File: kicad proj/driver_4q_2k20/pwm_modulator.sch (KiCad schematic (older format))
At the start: 9 parts, among them U2 LM555

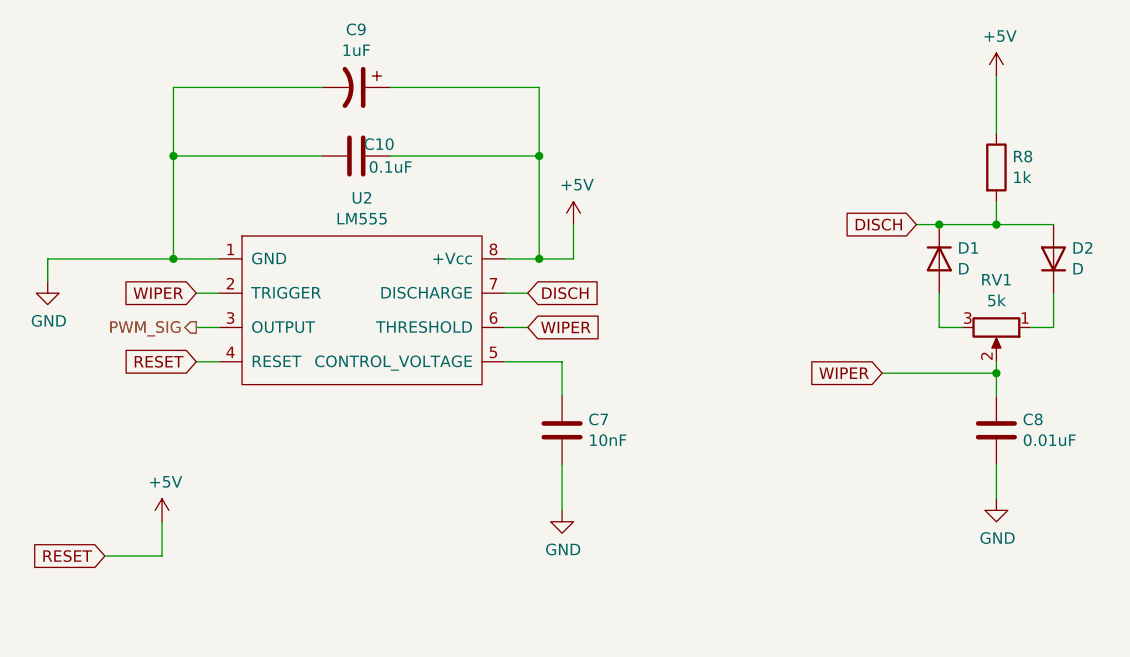
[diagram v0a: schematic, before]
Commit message: adicionado arquivos step, docs e footprints
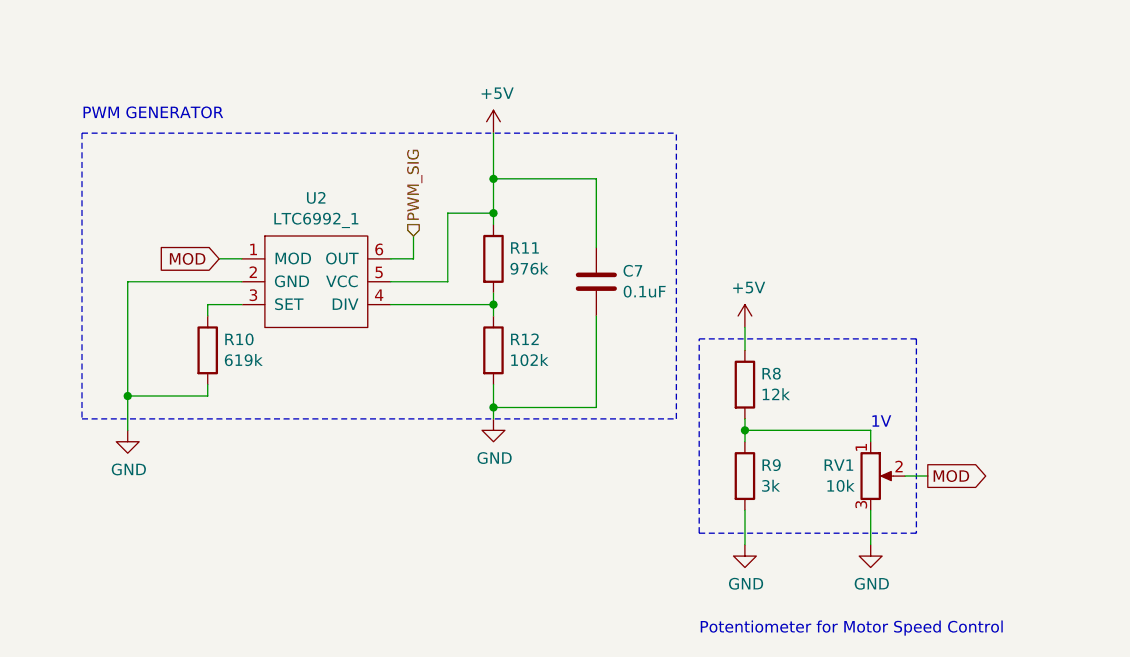
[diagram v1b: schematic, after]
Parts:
- removed C10: 0.1uF, driver_4q_2k20:C_0402_1005Metric, symbol Device:C
- removed C8: 0.01uF, driver_4q_2k20:C_0402_1005Metric, symbol Device:C
- removed C9: 1uF, driver_4q_2k20:CP_Radial_D5.0mm_P2.00mm, symbol Device:CP1
- removed D1, D2: D, driver_4q_2k20:S1_SMA, symbol Device:D
- removed U2: LM555, driver_4q_2k20:TI_DGN_S-PDSO-G8, symbol driver_4q_2k20_lib:555
- added R10: 619k, driver_4q_2k20:R_0402_1005Metric, symbol Device:R
- added R11: 976k, driver_4q_2k20:R_0402_1005Metric, symbol Device:R
- added R12: 102k, driver_4q_2k20:R_0402_1005Metric, symbol Device:R
- added R9: 3k, driver_4q_2k20:R_0402_1005Metric, symbol Device:R
- added U2: LTC6992_1, driver_4q_2k20:TSOT-23-6, symbol driver_4q_2k20_lib:LTC6992_1
- C7: value 10nF -> 0.1uF; Comment (none) -> ceramic / near LTC6992
- R8: value 1k -> 12k; footprint driver_4q_2k20:C_0402_1005Metric -> driver_4q_2k20:R_0402_1005Metric
- RV1: value 5k -> 10k
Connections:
- net DISCH is gone; now on an unnamed net: R8.2
- net +5V: now also C7.1, R11.1, U2.5 (VCC)
- net GND: now also RV1.3, R10.2, R12.2, R9.2, U2.2 (GND)
- net PWM_SIG: now also U2.6 (OUT)
- net at RV1.1: now also R9.1
- net WIPER renamed MOD
- net MOD: now also U2.1 (MOD)
- new net: R10.1, U2.3 (SET)
- new net: R11.2, R12.1, U2.4 (DIV)
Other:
- note added: "1V"
- note added: "PWM GENERATOR"
- note added: "Potentiometer for Motor Speed Control"
